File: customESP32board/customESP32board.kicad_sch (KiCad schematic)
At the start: 27 parts, among them J1 USB_B_Micro, J2 Conn_01x16_Pin, J3 Conn_01x16_Pin, Q1 S8050, Q2 S8050, SW1 SW_Push, SW2 SW_Push, U1 ESP32-WROOM-32, U2 CH340C, U3 AMS1117-3.3

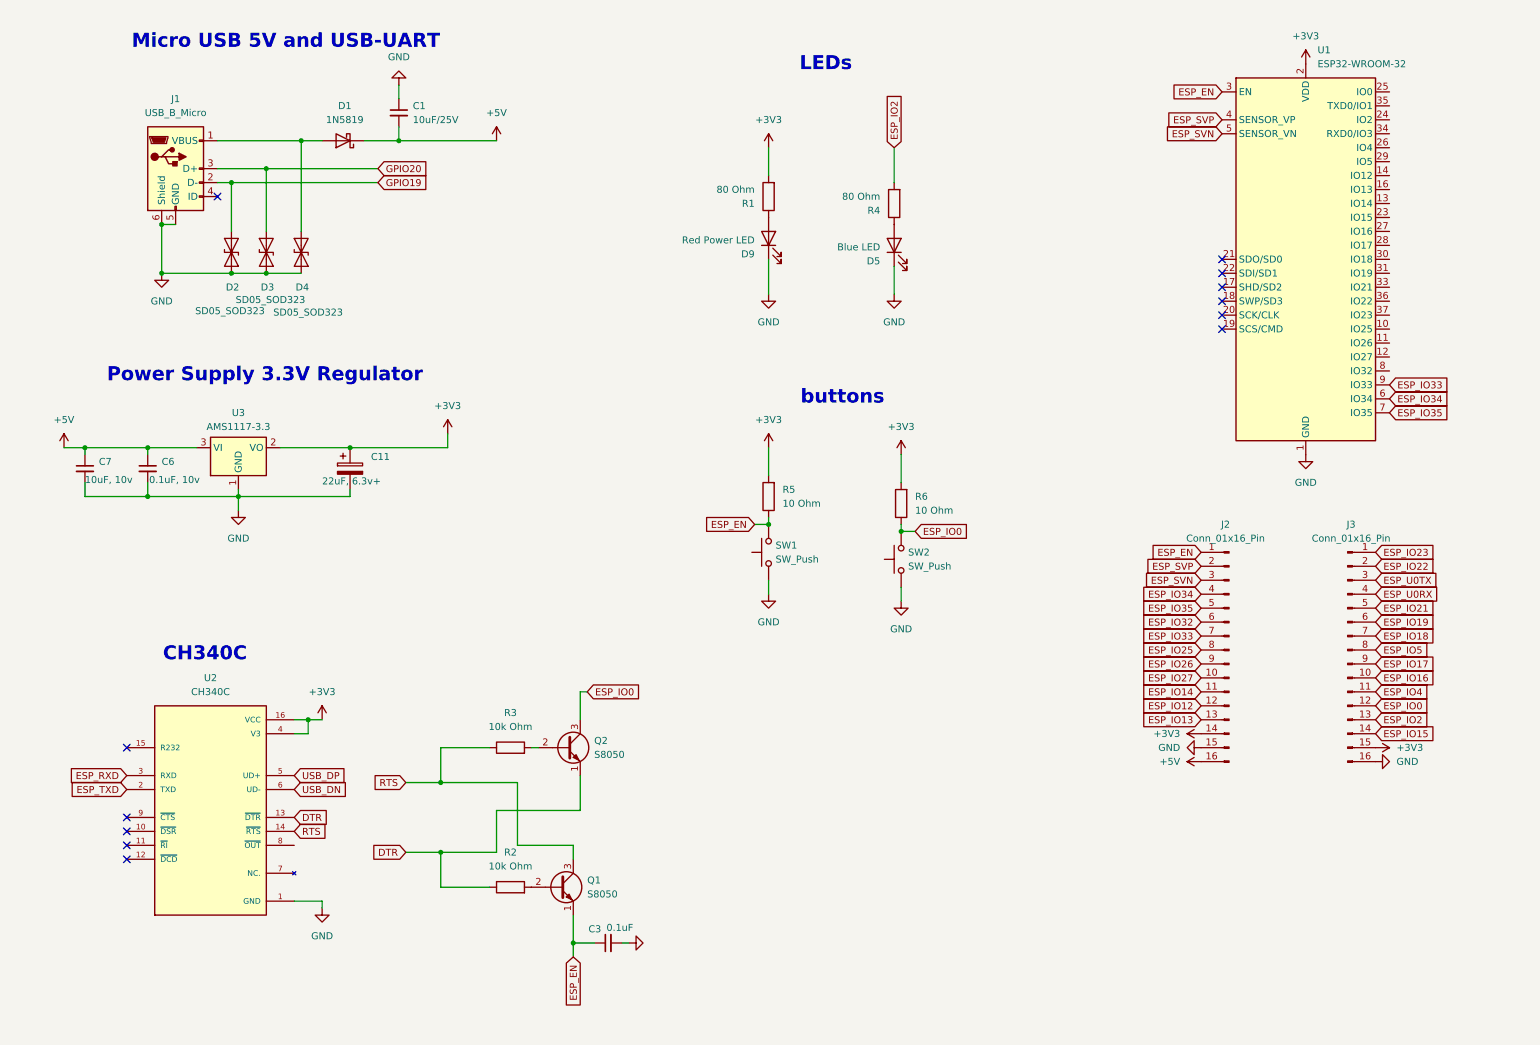
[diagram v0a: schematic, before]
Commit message: finalized esp32 board schematic
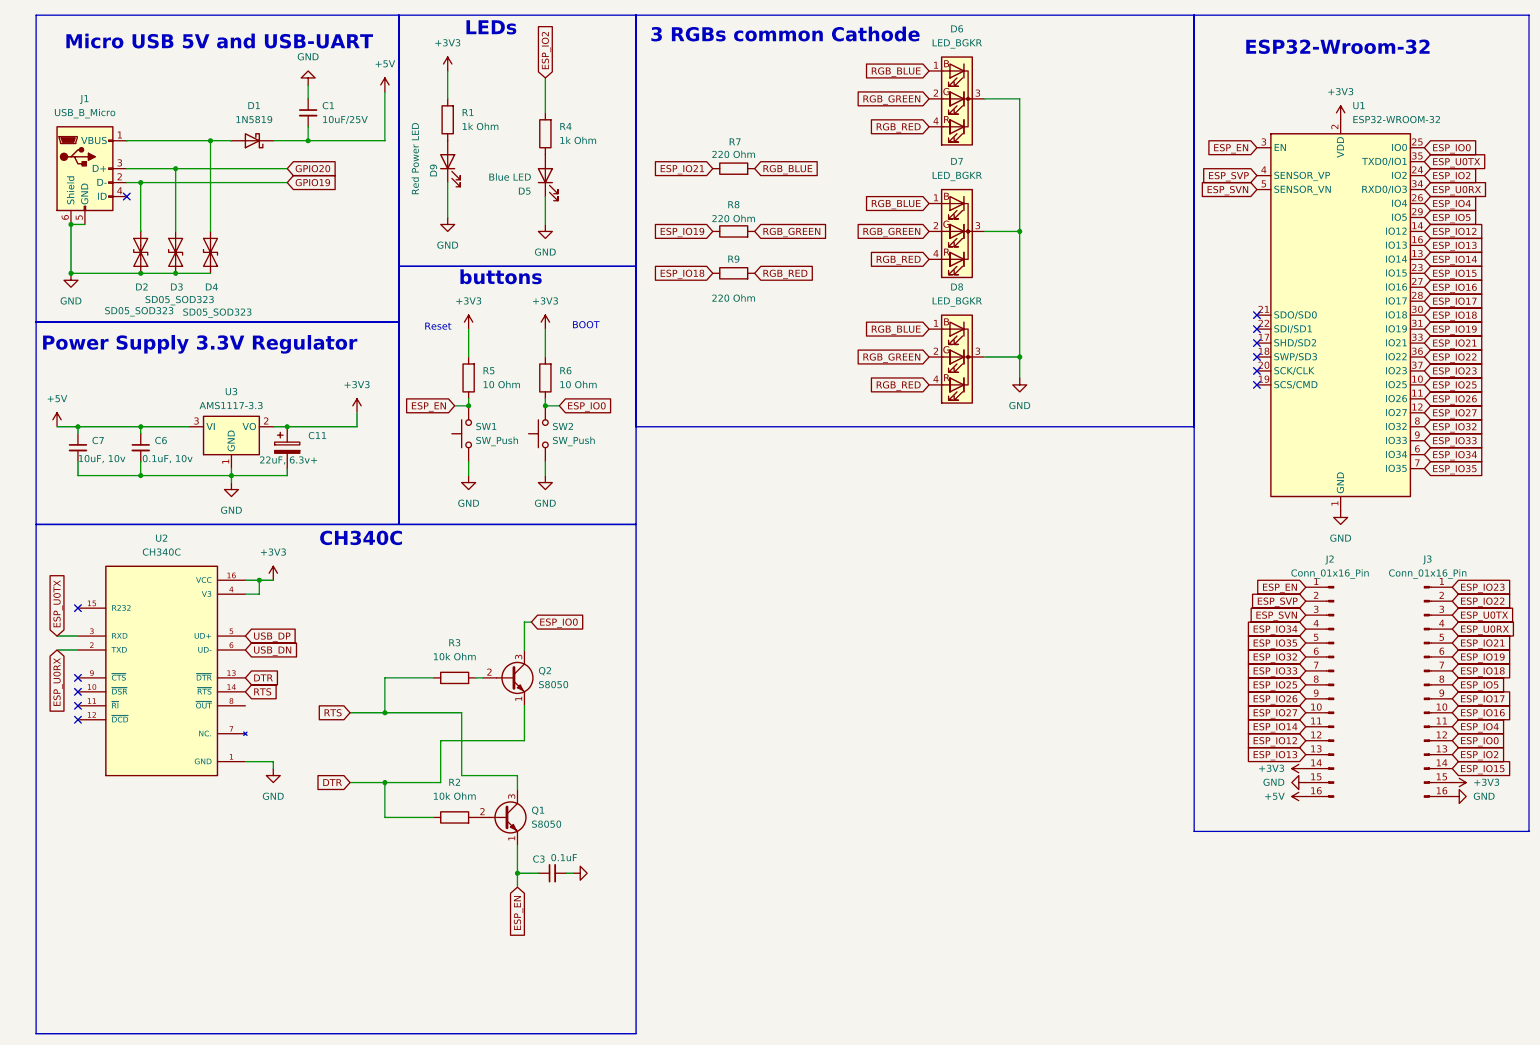
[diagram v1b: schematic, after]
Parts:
- added D6, D7, D8: LED_BGKR, symbol Device:LED_BGKR
- added R7, R8, R9: 220 Ohm, symbol Device:R
- R1, R4: value 80 Ohm -> 1k Ohm
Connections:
- net ESP_RXD is gone; now on net ESP_U0TX: U2.3 (RXD)
- net ESP_TXD is gone; now on net ESP_U0RX: U2.2 (TXD)
- net ESP_IO0: now also U1.25 (IO0)
- net ESP_IO12: now also U1.14 (IO12)
- net ESP_IO13: now also U1.16 (IO13)
- net ESP_IO14: now also U1.13 (IO14)
- net ESP_IO15: now also U1.23 (IO15)
- net ESP_IO16: now also U1.27 (IO16)
- net ESP_IO17: now also U1.28 (IO17)
- net ESP_IO18: now also U1.30 (IO18), R9.1
- net ESP_IO19: now also U1.31 (IO19), R8.1
- net ESP_IO2: now also U1.24 (IO2)
- net ESP_IO21: now also U1.33 (IO21), R7.1
- net ESP_IO22: now also U1.36 (IO22)
- net ESP_IO23: now also U1.37 (IO23)
- net ESP_IO25: now also U1.10 (IO25)
- net ESP_IO26: now also U1.11 (IO26)
- net ESP_IO27: now also U1.12 (IO27)
- net ESP_IO32: now also U1.8 (IO32)
- net ESP_IO4: now also U1.26 (IO4)
- net ESP_IO5: now also U1.29 (IO5)
- net ESP_U0RX: now also U1.34 (RXD0/IO3)
- net ESP_U0TX: now also U1.35 (TXD0/IO1)
- net GND: now also D6.3 (K), D7.3 (K), D8.3 (K)
- new net RGB_BLUE: D6.1 (BA), D7.1 (BA), D8.1 (BA), R7.2
- new net RGB_GREEN: D6.2 (GA), D7.2 (GA), D8.2 (GA), R8.2
- new net RGB_RED: D6.4 (RA), D7.4 (RA), D8.4 (RA), R9.2
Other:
- note added: "3 RGBs common Cathode"
- note added: "BOOT"
- note added: "ESP32-Wroom-32"
- note added: "Reset"
- moved on the sheet: C1, C11, C3, C6, C7, D1, D2, D3, D4, D5, D9, J1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
